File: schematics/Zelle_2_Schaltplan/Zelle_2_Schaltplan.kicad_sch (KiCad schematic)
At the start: 14 parts, among them J1 Raspberry_Pi_4, K1 12V Relais, M1 Pumpe, U1 ESP32-WROOM-32U, U2 DS18B20, U3 DS18B20

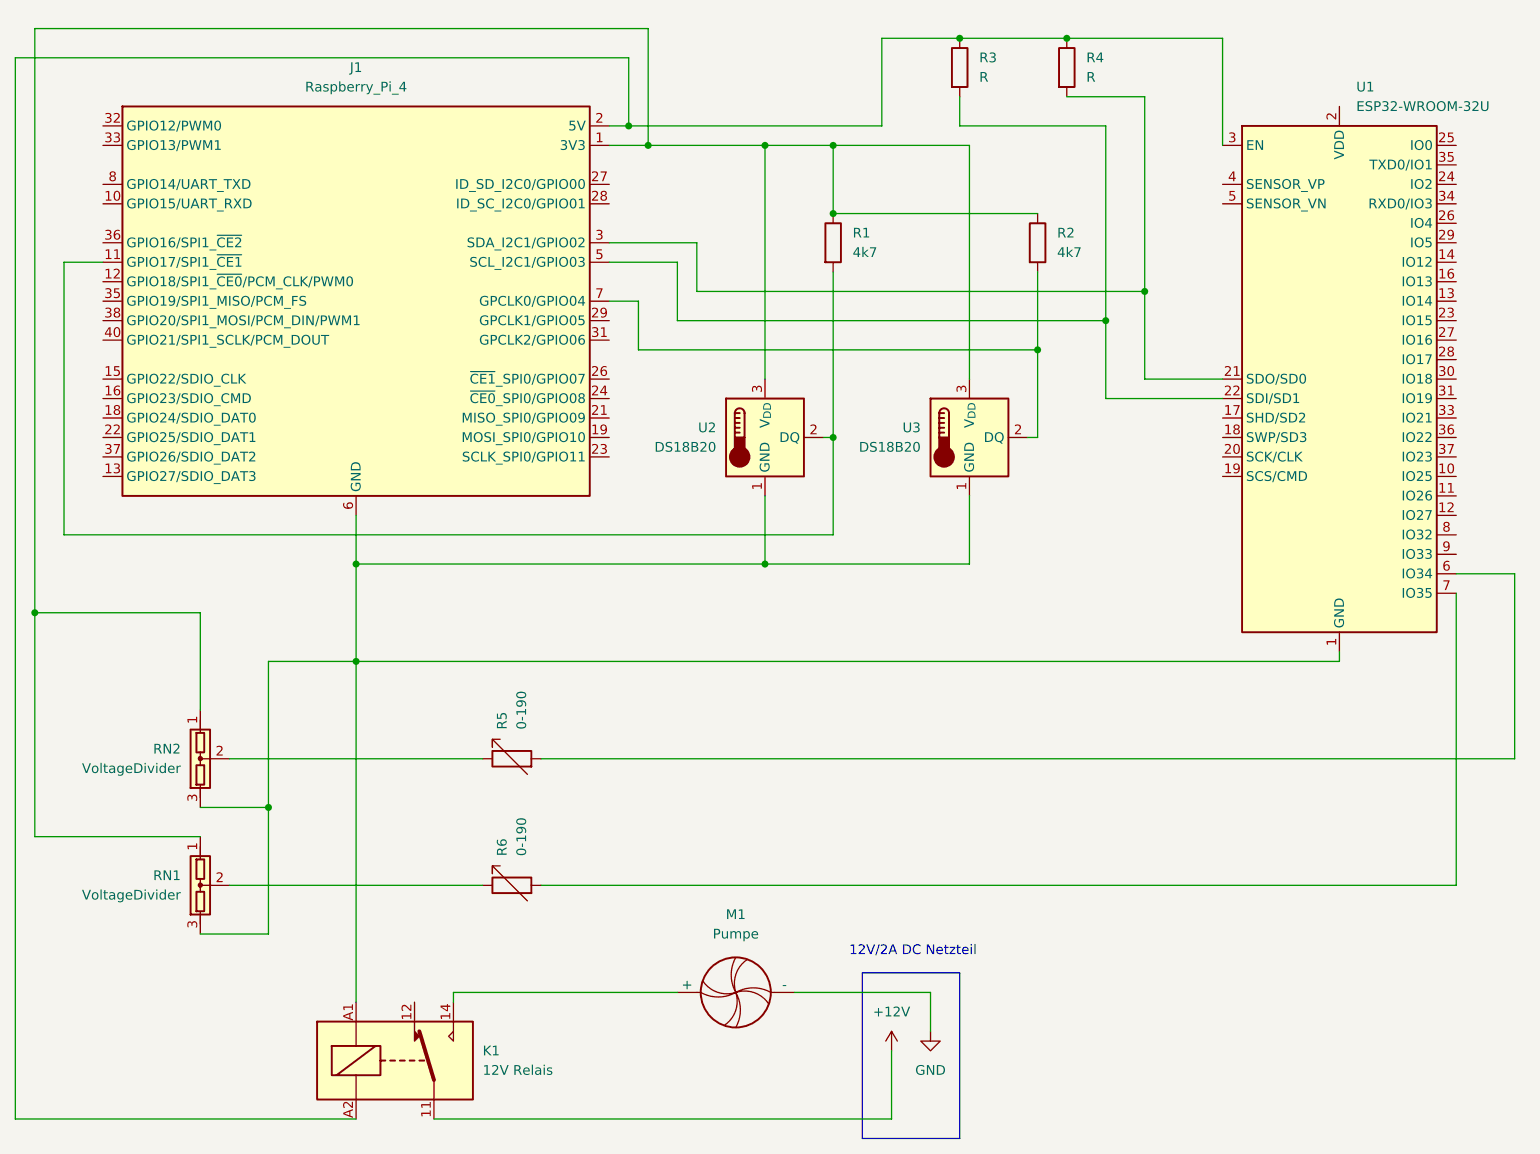
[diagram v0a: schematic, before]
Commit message: 2. Schaltplan überarbeitet
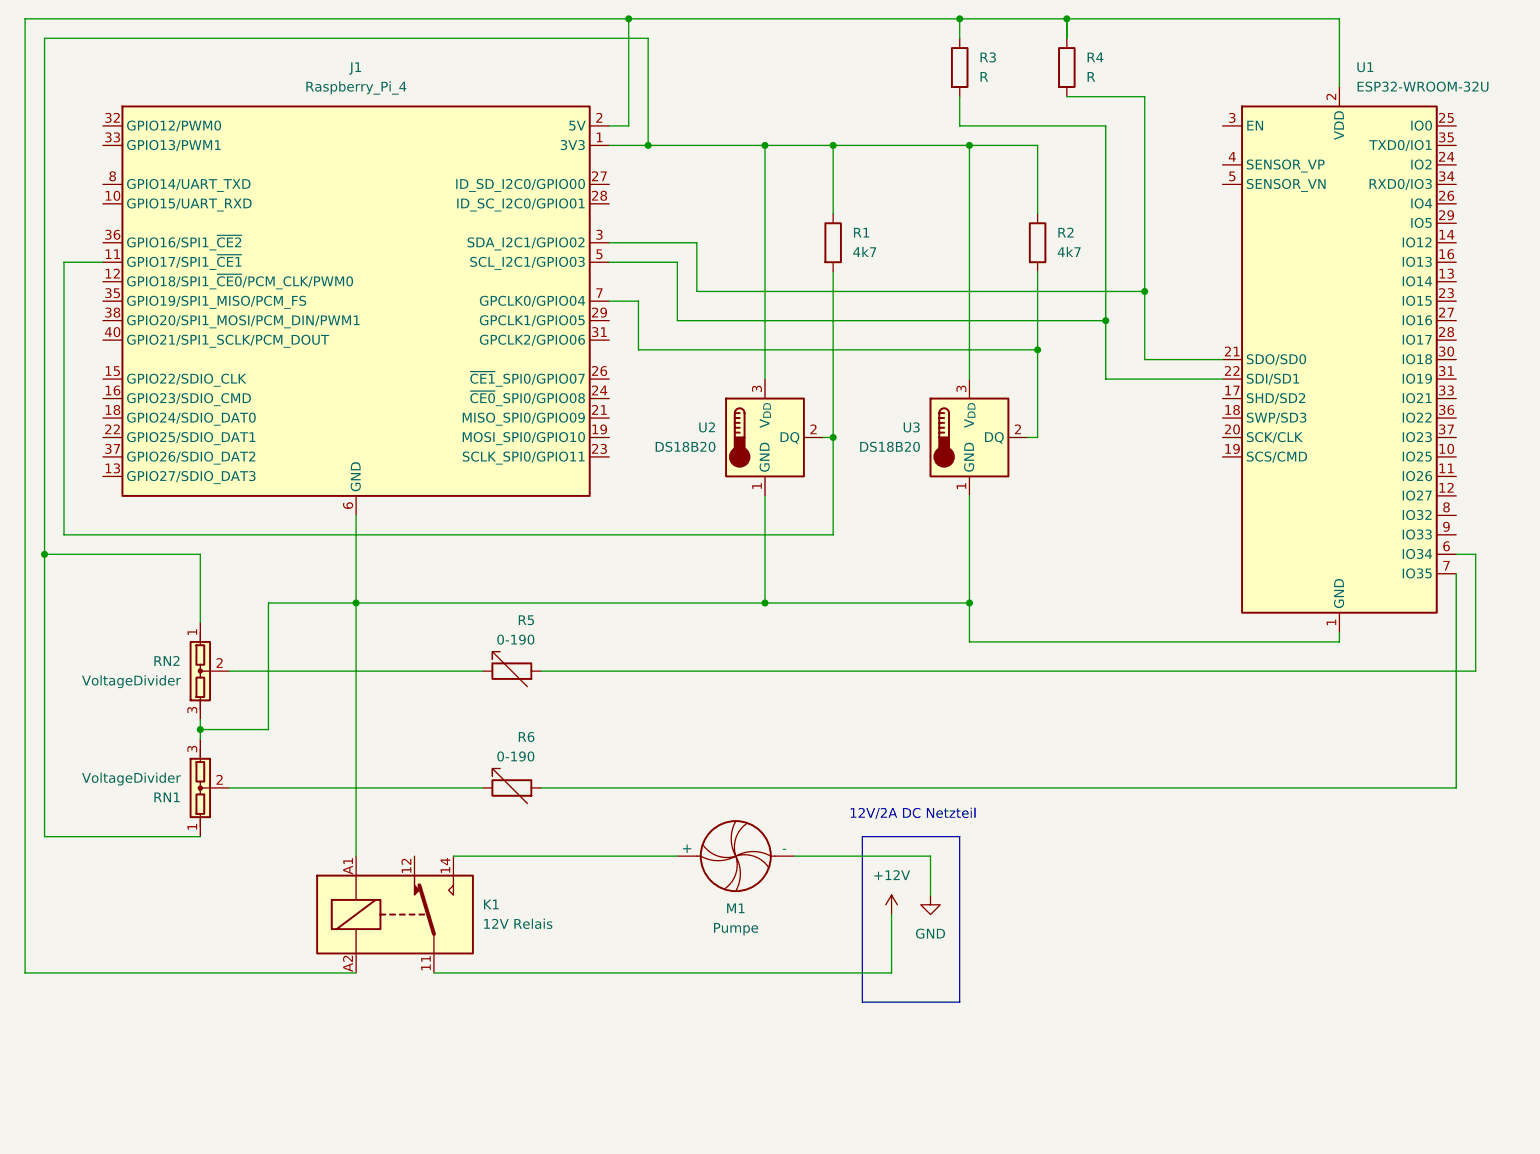
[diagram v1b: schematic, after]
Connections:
- net at U1.2 (VDD): now also J1.2 (5V), J1.4 (5V), K1.A2, R3.1, R4.1
- now unconnected: U1.3 (EN)
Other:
- moved on the sheet: K1, M1, R5, R6, RN1, RN2, U1
